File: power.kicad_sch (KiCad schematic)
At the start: 21 parts, among them U10 RT9080-33GJ5, U11 AP22804AW5, U8 TPS2120YFPR, U9 RT9080-33GJ5

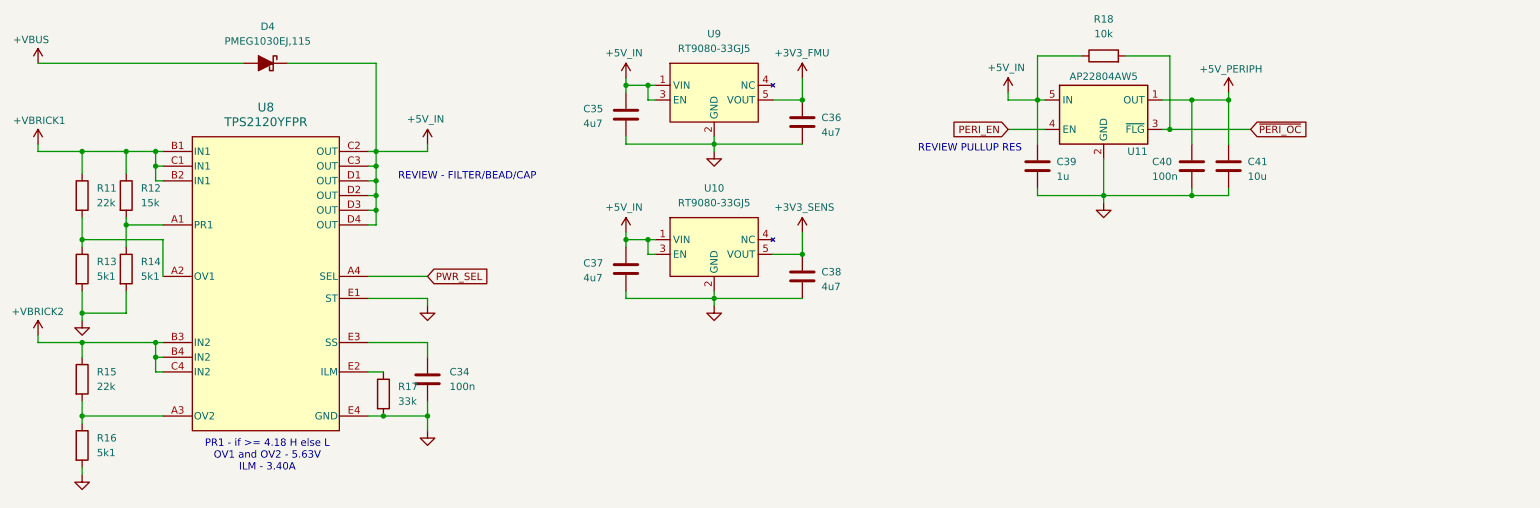
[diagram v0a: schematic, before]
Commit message: Mulai layout
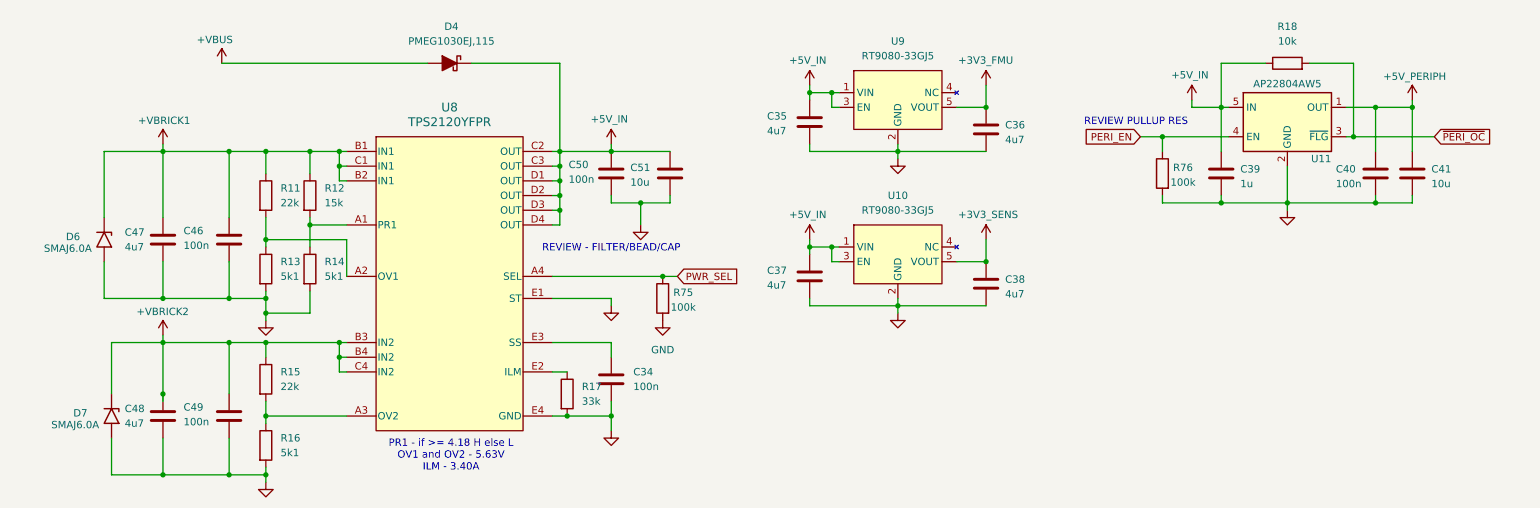
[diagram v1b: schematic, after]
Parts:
- added C46, C49, C50: 100n, Capacitor_SMD:C_0402_1005Metric, symbol Device:C
- added C47, C48: 4u7, Capacitor_SMD:C_0603_1608Metric, symbol Device:C
- added C51: 10u, Capacitor_SMD:C_0603_1608Metric, symbol Device:C
- added D6, D7: SMAJ6.0A, Diode_SMD:D_SMA, symbol Diode:SMAJ6.0A
- added R75, R76: 100k, Resistor_SMD:R_0402_1005Metric, symbol Device:R
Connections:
- net +5V_IN: now also C50.1, C51.1
- net +VBRICK1: now also C46.1, C47.1, D6.1 (A1)
- net +VBRICK2: now also C48.1, C49.1, D7.1 (A1)
- net GND: now also C46.2, C47.2, C48.2, C49.2, C50.2, C51.2, D6.2 (A2), D7.2 (A2), R75.2, R76.2
- net PERI_EN: now also R76.1
- net PWR_SEL: now also R75.1
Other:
- moved on the sheet: C34, C35, C36, C37, C38, C39, C40, C41, D4, R11, R12, R13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
